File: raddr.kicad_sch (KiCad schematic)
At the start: 6 parts, among them J1 Conn_01x04, J3 Conn_01x04, U1 PMS150C-U06

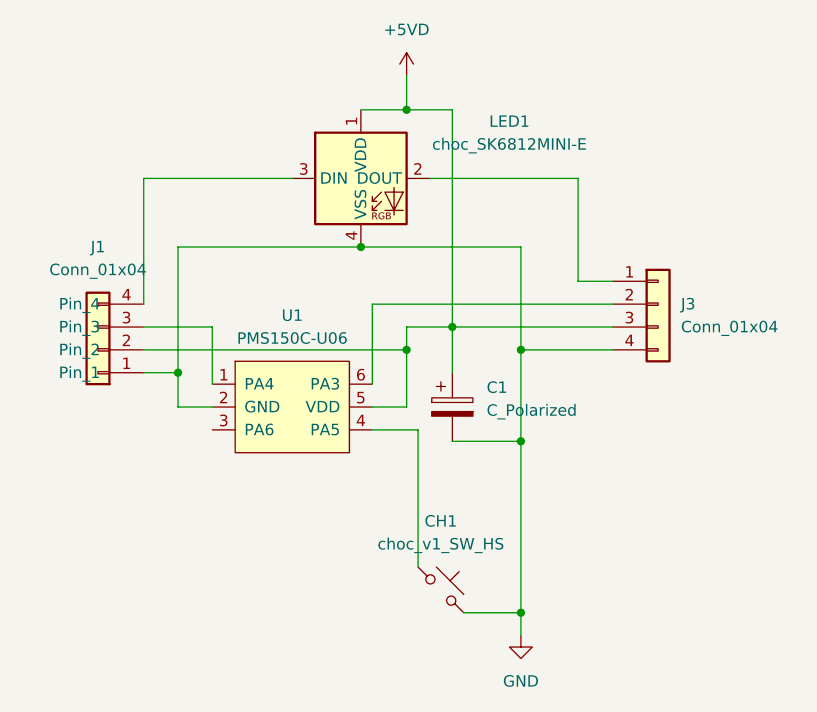
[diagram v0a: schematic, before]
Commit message: add traces
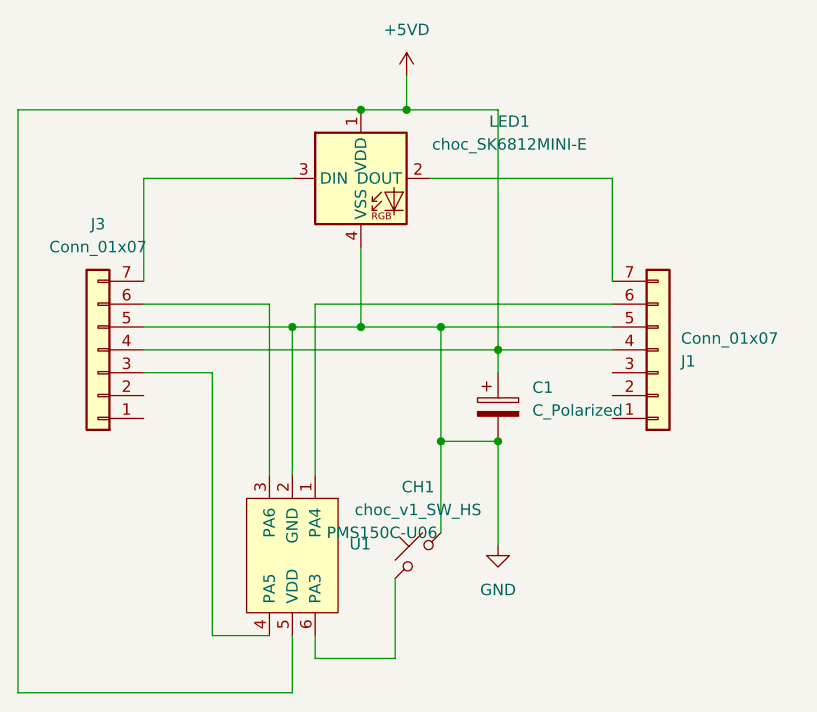
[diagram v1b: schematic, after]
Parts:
- removed J1, J3: Conn_01x04, Connector_PinSocket_2.54mm:PinSocket_1x04_P2.54mm_Vertical, symbol Connector_Generic:Conn_01x04
- added J1, J3: Conn_01x07, Connector_PinSocket_2.54mm:PinSocket_1x07_P2.54mm_Vertical, symbol Connector_Generic:Conn_01x07
- C1: footprint Capacitor_SMD:C_0402_1005Metric -> Capacitor_SMD:C_0603_1608Metric_Pad1.08x0.95mm_HandSolder
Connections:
- net +5VD: now also J1.4 (Pin_4), J3.4 (Pin_4)
- net GND: now also CH1.1, J1.5 (Pin_5), J3.5 (Pin_5); no longer CH1.2
- net at LED1.2 (DOUT): now also J1.7 (Pin_7)
- net at LED1.3 (DIN): now also J3.7 (Pin_7)
- net at U1.1 (PA4): now also J1.6 (Pin_6)
- net at U1.6 (PA3): now also CH1.2
- net at U1.3 (PA6): now also J3.6 (Pin_6)
- net at U1.4 (PA5): now also J3.3 (Pin_3); no longer CH1.1
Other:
- moved on the sheet: C1, CH1, U1
